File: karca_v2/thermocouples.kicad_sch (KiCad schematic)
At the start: 13 parts, among them J8 Screw_Terminal_01x08, U12 NUP4202, U13 TLV9304xD

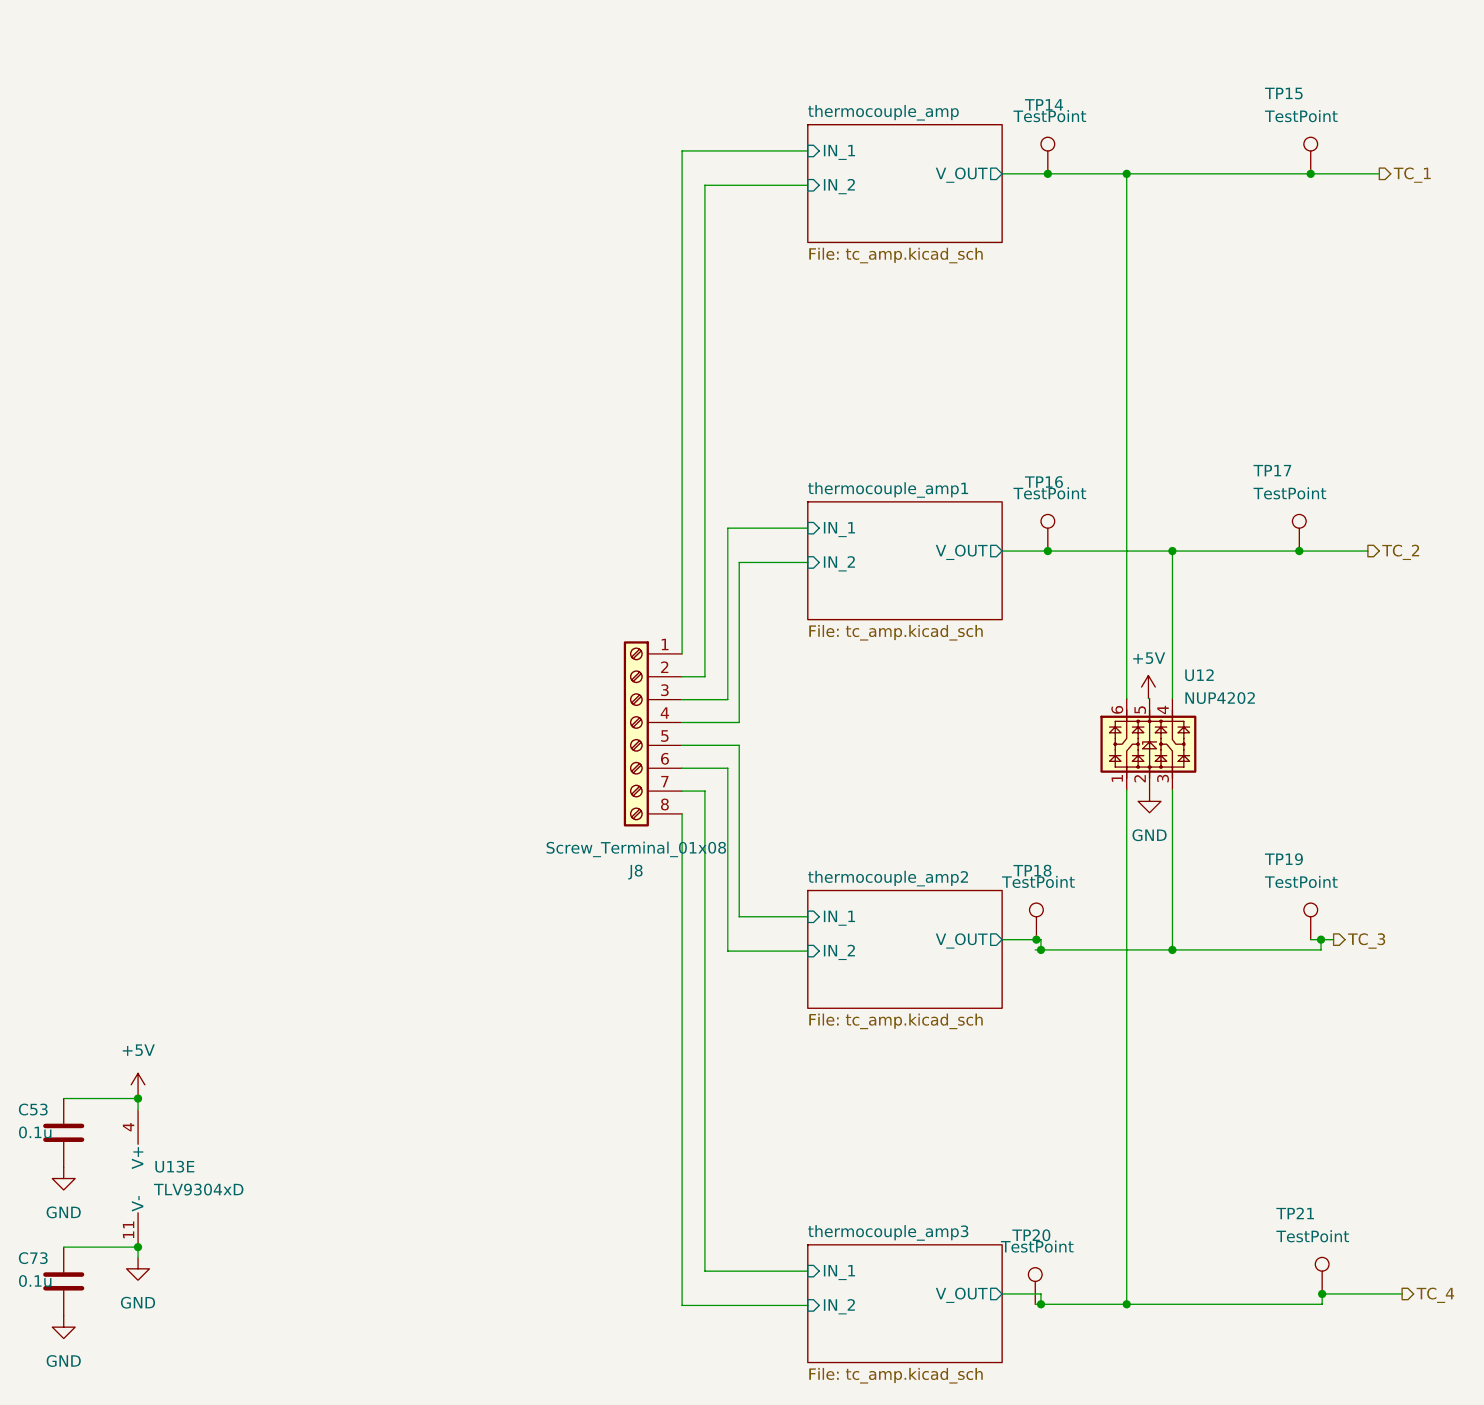
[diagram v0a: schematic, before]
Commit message: fkkkkkkkkkk
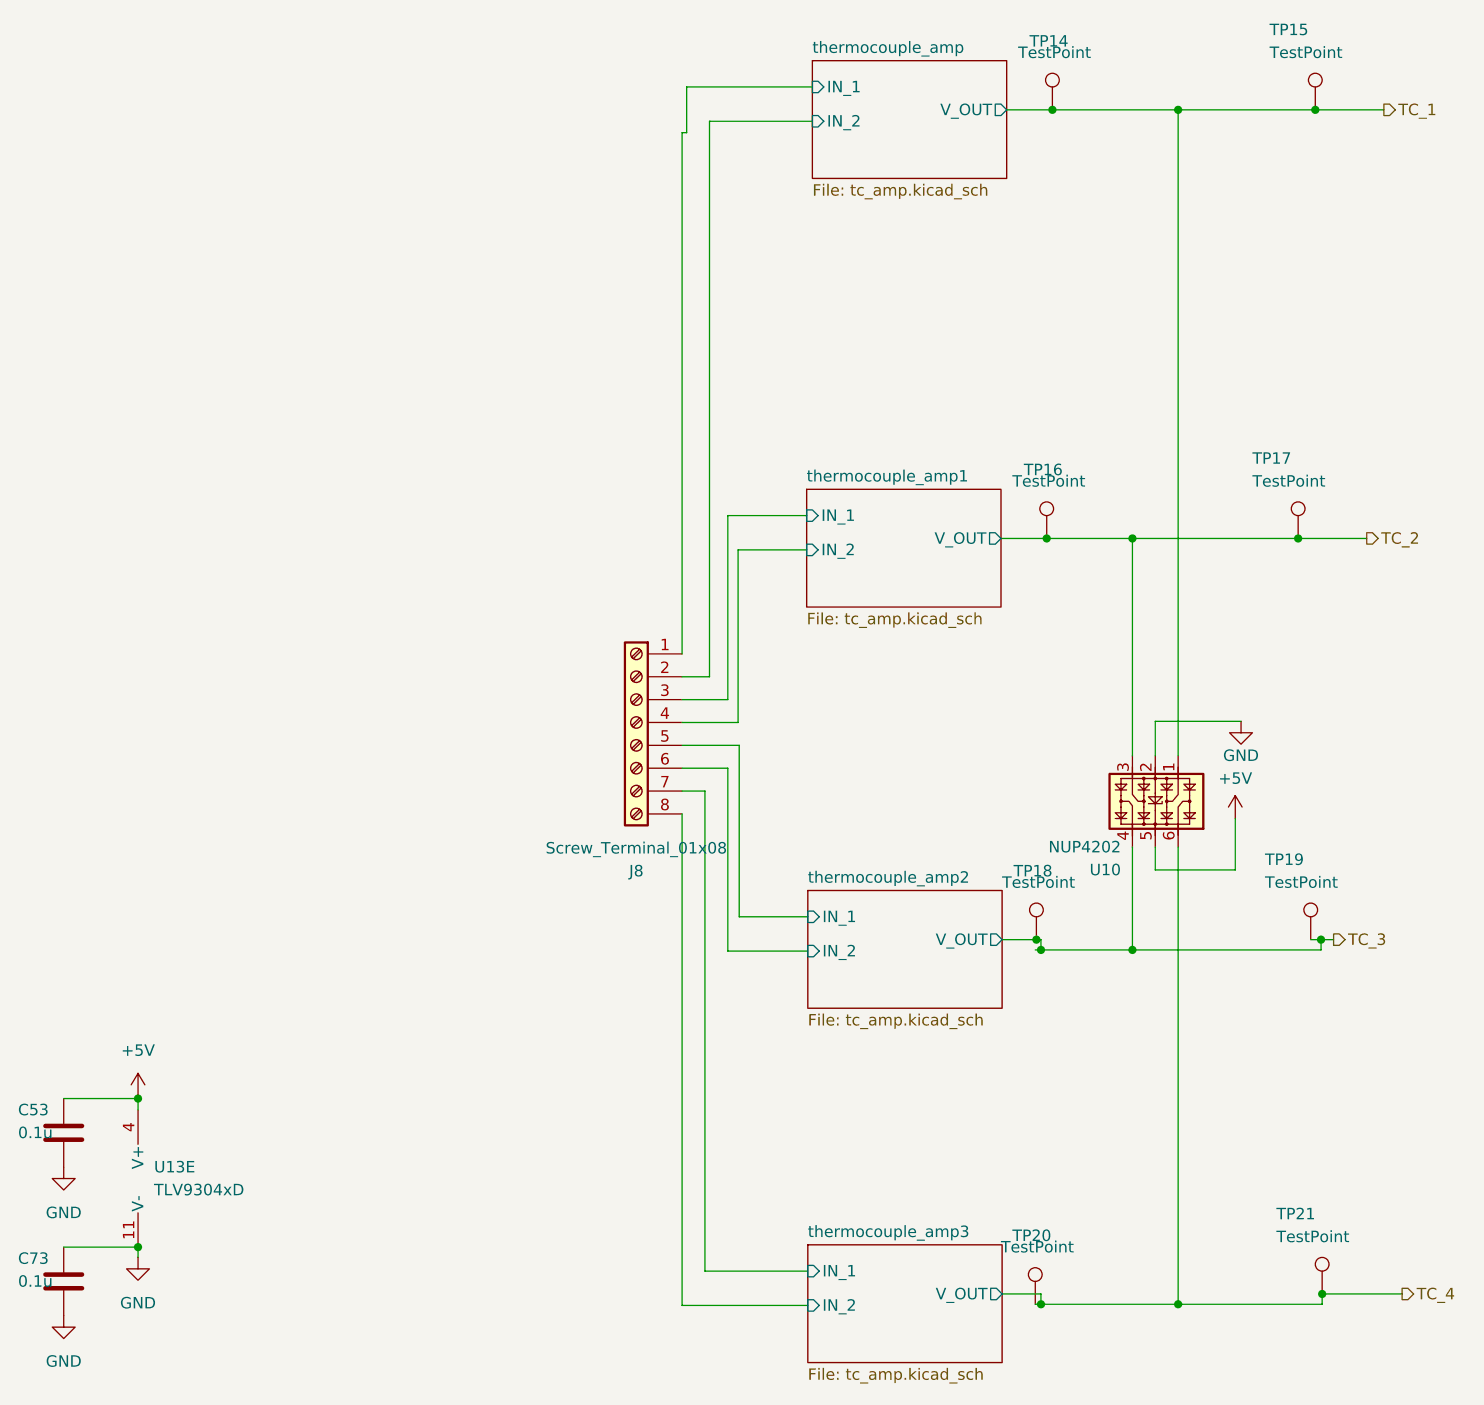
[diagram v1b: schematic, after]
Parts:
- U10: renamed from U12; footprint Package_SO:TSOP-6_1.65x3.05mm_P0.95mm -> Package_TO_SOT_SMD:SOT-363_SC-70-6
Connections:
- net TC_1: now also U10.1; no longer U10.6
- net TC_2: now also U10.3; no longer U10.4
- net TC_3: now also U10.4; no longer U10.3
- net TC_4: now also U10.6; no longer U10.1
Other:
- moved on the sheet: TP14, TP15, TP16, TP17, U10
